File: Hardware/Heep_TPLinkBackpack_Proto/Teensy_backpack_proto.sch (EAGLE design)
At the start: 30 parts, among them Q1 25MHz, Q2 600mA/40V, U1 ENC28J60-SO

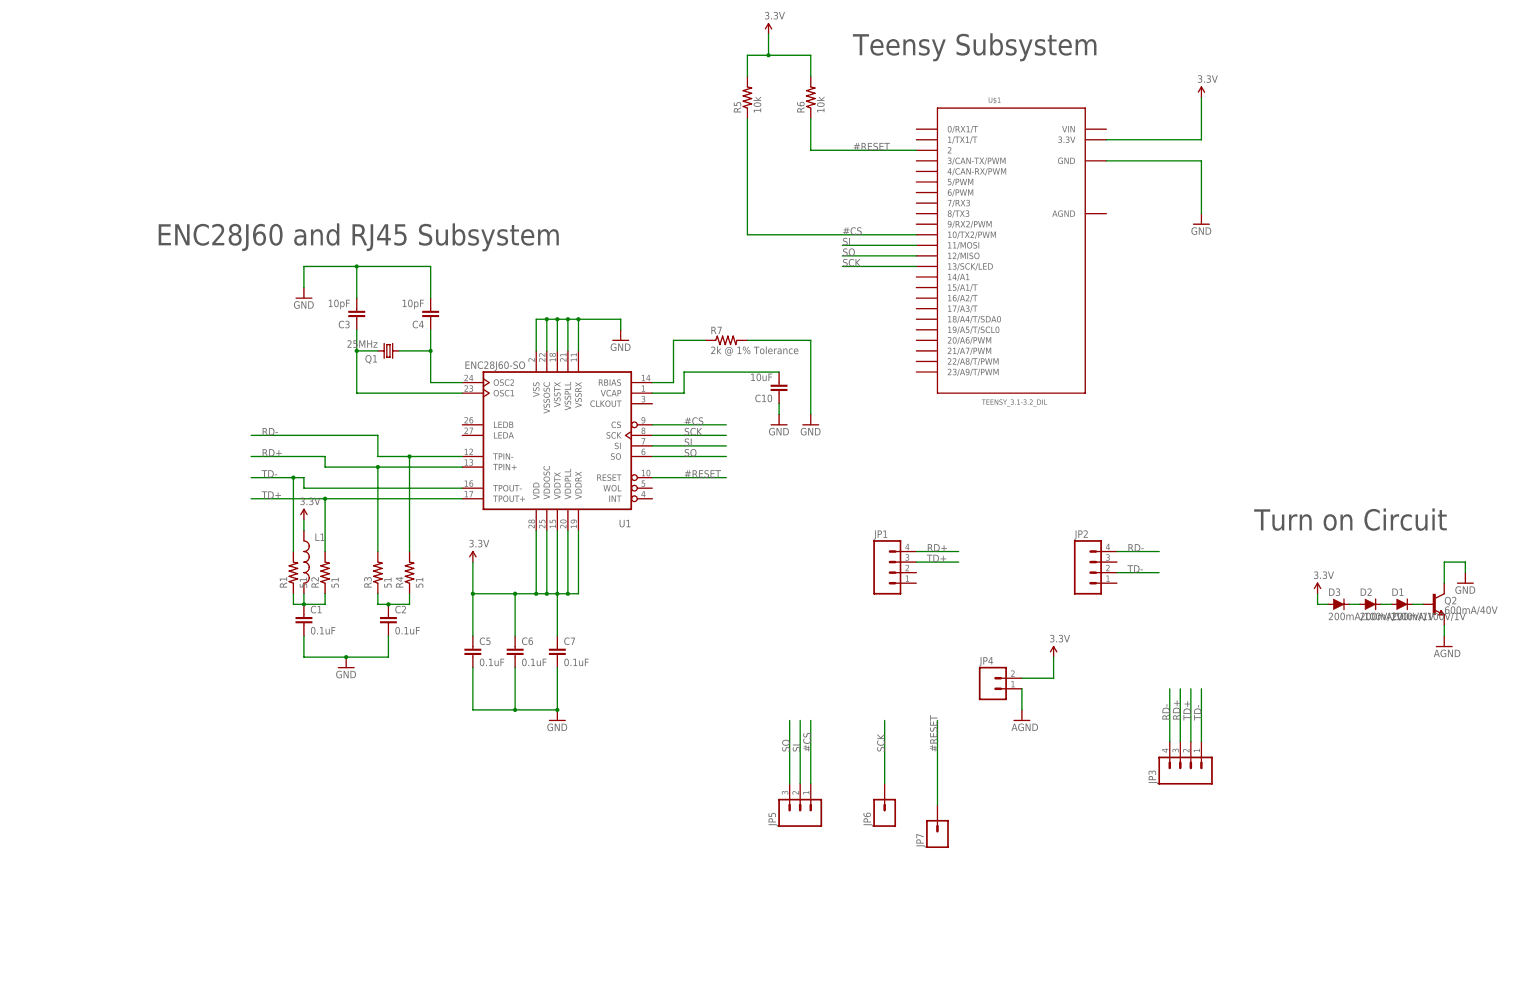
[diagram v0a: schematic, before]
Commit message: #44 almost done with board design
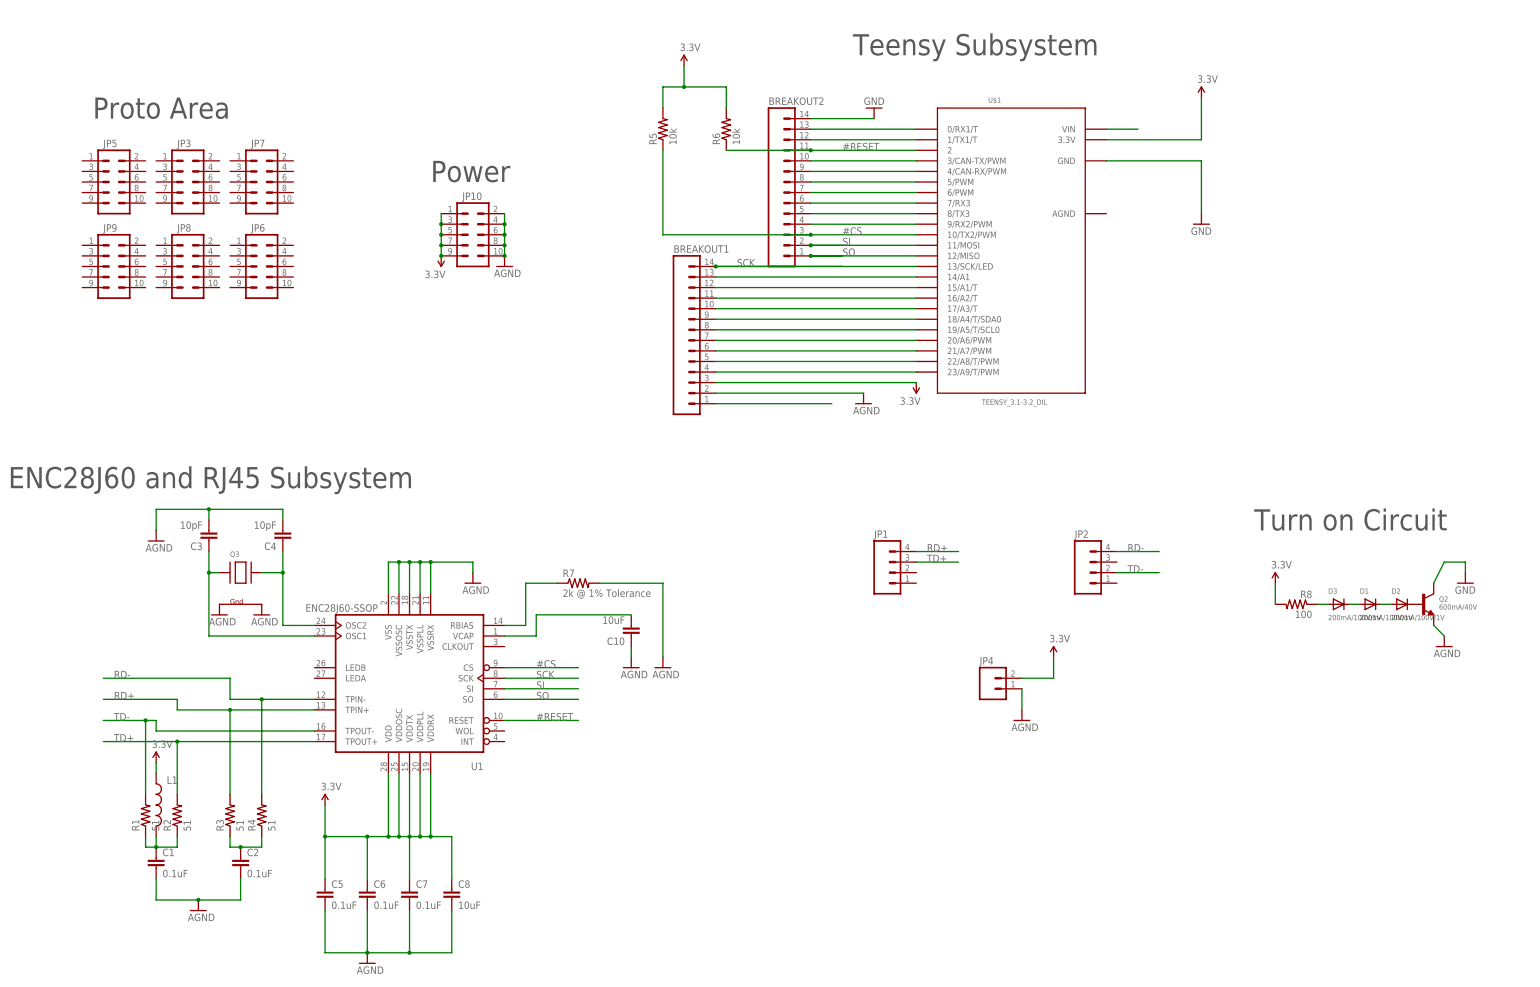
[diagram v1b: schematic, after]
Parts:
- removed Q1: 25MHz, adafruit:CRYSTALSM49
- added BREAKOUT1, BREAKOUT2: (no value), SparkFun-Connectors:M14
- added C8: 10uF, SparkFun-Passives:CAP0603-CAP
- added JP10, JP8, JP9: (no value), SparkFun-Connectors:M05X2NO_SILK
- added Q3: (no value), adafruit:XTAL-4-3225
- added R8: 100, SparkFun-Resistors:RESISTOR0603
- D1, D2, D3: device SparkFun-DiscreteSemi:DIODE-1N4148 -> adafruit:DIODESOD-123
- JP3: device SparkFun-Connectors:M04NO_SILK_ALL_ROUND -> SparkFun-Connectors:M05X2NO_SILK
- JP5: device SparkFun-Connectors:M03PTH -> SparkFun-Connectors:M05X2NO_SILK
- JP6, JP7: device SparkFun-Connectors:M01PTH -> SparkFun-Connectors:M05X2NO_SILK
- Q2: device SparkFun-DiscreteSemi:TRANS_NPN-P2N2222A -> microbuilder:TRANSISTOR_NPN
- U1: value ENC28J60-SO -> ENC28J60-SSOP; device microchip-enc28j60:ENC28J60-SO -> microchip-enc28j60:ENC28J60-SSOP
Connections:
- new net N$10: BREAKOUT2.7, U$1.6/PWM
- new net N$11: BREAKOUT2.8, U$1.5/PWM
- new net N$14: BREAKOUT2.9, U$1.4/CAN-RX/PWM
- new net N$16: BREAKOUT2.10, U$1.3/CAN-TX/PWM
- new net N$18: BREAKOUT2.12, U$1.1/TX1/T
- new net N$19: BREAKOUT2.13, U$1.0/RX1/T
- new net N$20: BREAKOUT1.4, U$1.23/A9/T/PWM
- new net N$21: BREAKOUT1.5, U$1.22/A8/T/PWM
- new net N$22: BREAKOUT1.6, U$1.21/A7/PWM
- new net N$23: BREAKOUT1.7, U$1.20/A6/PWM
- new net N$24: BREAKOUT1.8, U$1.19/A5/T/SCL0
- new net N$25: BREAKOUT1.9, U$1.18/A4/T/SDA0
- new net N$26: BREAKOUT1.10, U$1.17/A3/T
- new net N$27: BREAKOUT1.11, U$1.16/A2/T
- new net N$28: BREAKOUT1.12, U$1.15/A1/T
- new net N$29: BREAKOUT1.13, U$1.14/A1
- new net N$4: D3.A, R8.1
- new net N$6: BREAKOUT2.4, U$1.9/RX2/PWM
- new net N$8: BREAKOUT2.5, U$1.8/TX3
- new net N$9: BREAKOUT2.6, U$1.7/RX3
- new net TEENSY_VIN: BREAKOUT1.1, U$1.VIN
- net #CS: now also BREAKOUT2.3; no longer JP5.1
- net #RESET: now also BREAKOUT2.11; no longer JP7.1
- net 3.3V: now also BREAKOUT1.3, C8.1, JP10.1, JP10.3, JP10.5, JP10.7, JP10.9, R8.2; no longer D3.A
- net AGND: now also BREAKOUT1.2, C1.2, C10.1, C2.2, C3.2, C4.2, C5.2, C6.2, C7.2, C8.2, JP10.10, JP10.2, JP10.4, JP10.6, JP10.8, Q3.G1, Q3.G2, R7.2, U1.VSS, U1.VSSOSC, U1.VSSPLL, U1.VSSRX, U1.VSSTX
- net GND: now also BREAKOUT2.14; no longer C1.2, C10.1, C2.2, C3.2, C4.2, C5.2, C6.2, C7.2, R7.2, U1.VSS, U1.VSSOSC, U1.VSSPLL, U1.VSSRX, U1.VSSTX
- net N$1: now also D1.C, D2.A; no longer D1.A, D2.C
- net N$12: now also Q3.X1; no longer Q1.2
- net N$13: now also Q3.X2; no longer Q1.1
- net N$2: now also D2.C; no longer D1.C
- net N$3: now also D1.A; no longer D2.A
- net RD+: no longer JP3.3
- net RD-: no longer JP3.4
- net SCK: now also BREAKOUT1.14; no longer JP6.1
- net SI: now also BREAKOUT2.2; no longer JP5.2
- net SO: now also BREAKOUT2.1; no longer JP5.3
- net TD+: no longer JP3.2
- net TD-: no longer JP3.1
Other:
- note added: "Power"
- note added: "Proto Area"
- moved on the sheet: C1, C10, C2, C3, C4, C5, C6, C7, L1, Q2, R1, R2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
